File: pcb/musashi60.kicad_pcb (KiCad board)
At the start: 2 copper layers, 185 x 132 mm, 77 parts, among them J1 MJ-4PP-9, U1 ProMicro_r

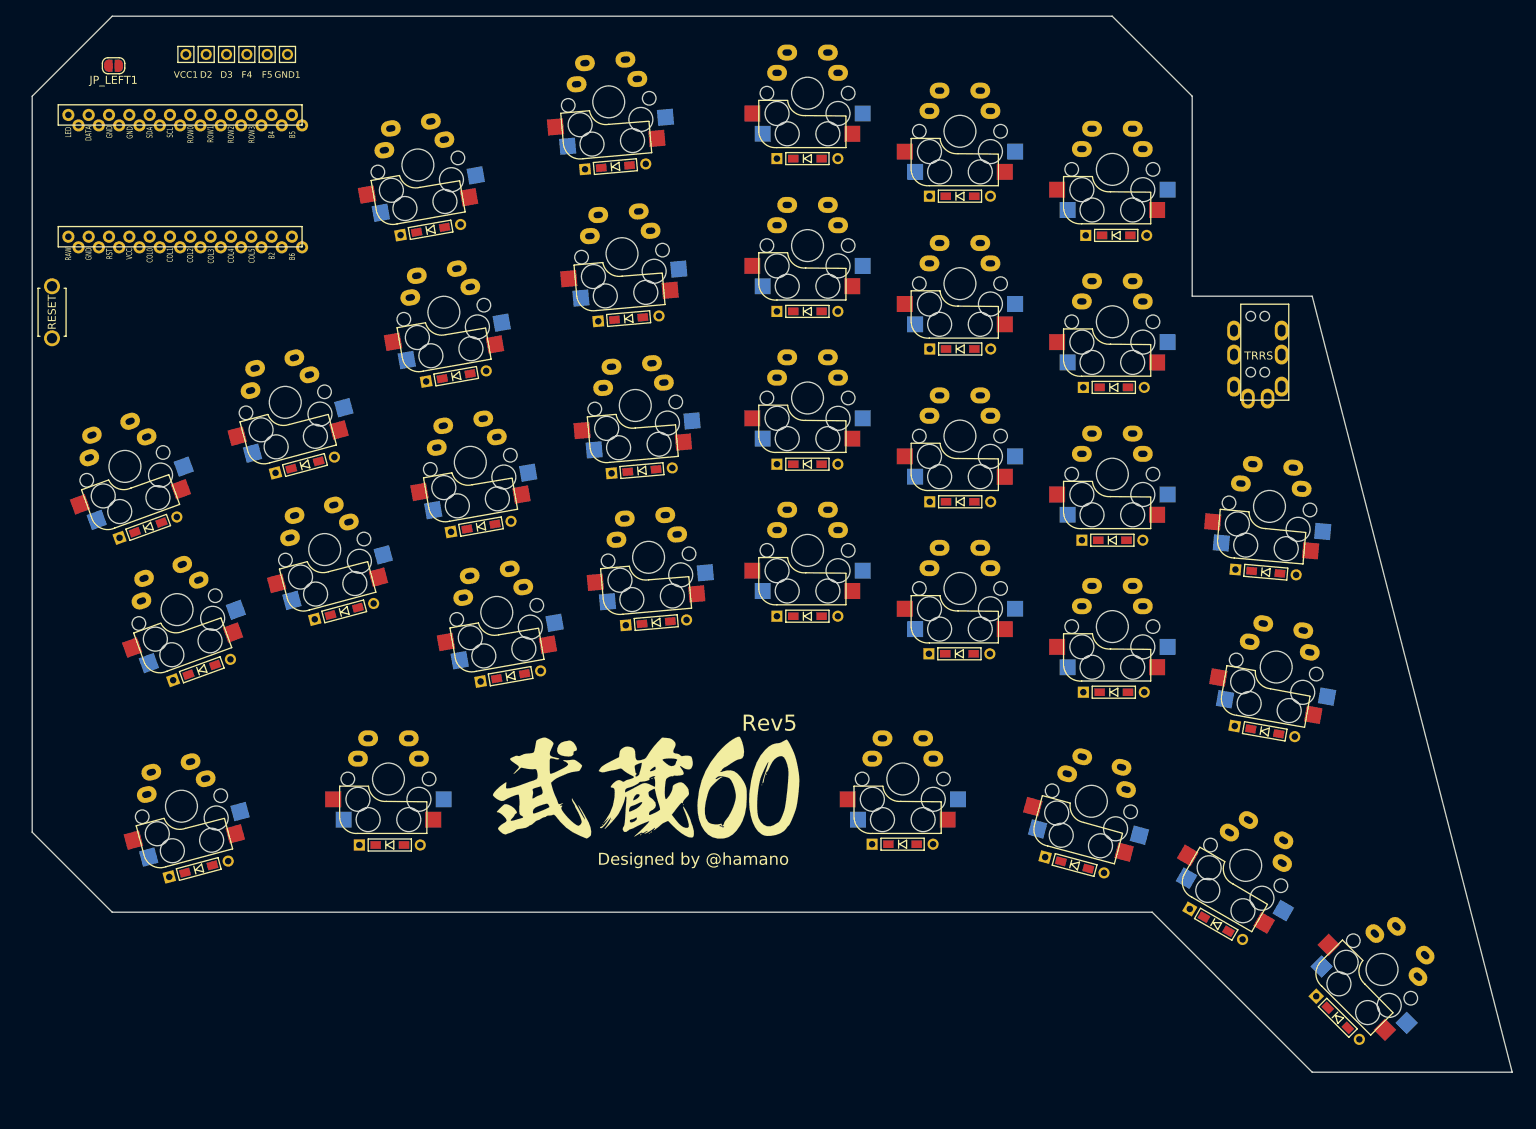
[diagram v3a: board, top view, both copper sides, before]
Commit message: update pcb
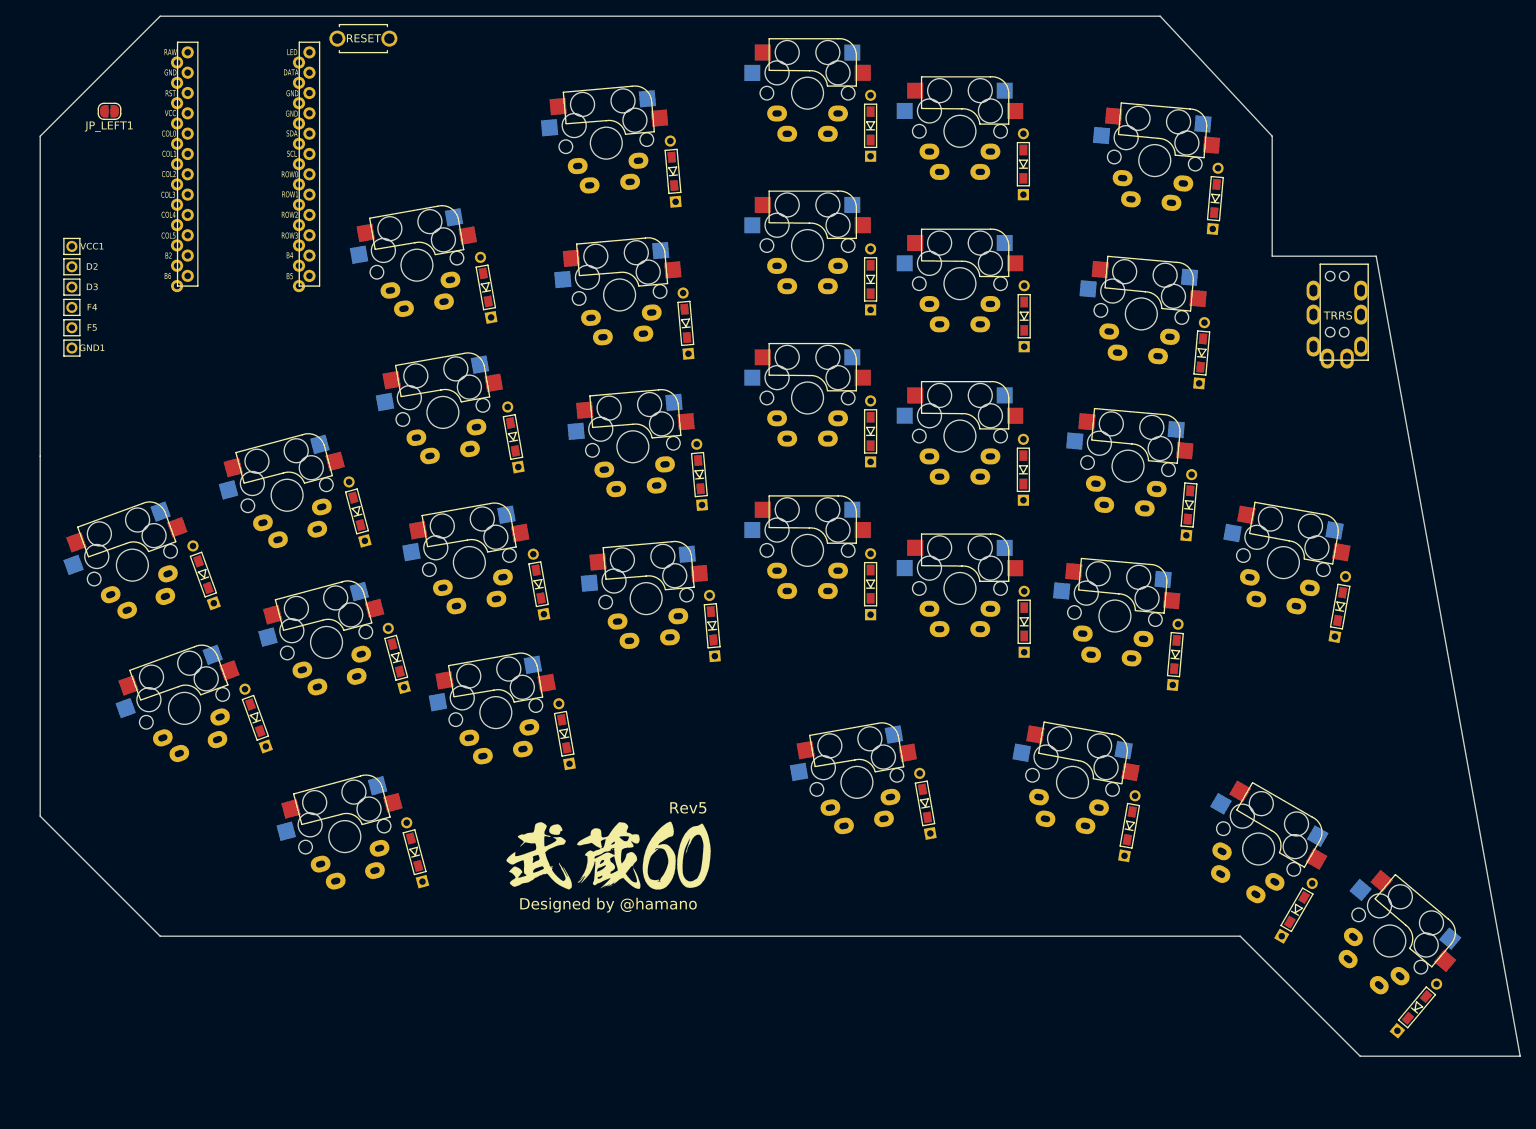
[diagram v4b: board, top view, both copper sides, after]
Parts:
- removed the D_A3 at (169.2, 82.5)
- removed D_H4: D, foostan:D3_TH_SMD
- removed the G_LOGO_B at (91.7, 109.4)
- removed the G_LOGO_F at (91.7, 109.5)
- removed the SW_A3 at (169.7, 74.3)
- removed SW_H4: SW_PUSH, local:CherryMX_Direct_Hotswap_Reversible
- added G_LOGO_B: LOGO, local:musashi60-silk-384, B.Cu at (87.0, 118.0)
- added G_LOGO_F: LOGO, local:musashi60-silk-384, F.Cu at (87.0, 118.0)
- moved SW_RST1 51.8 mm to (56.4, 15.8), turned to 0 degrees
- moved GND1 45.5 mm to (20.0, 54.5)
- moved F5 42.0 mm to (20.0, 51.9)
- moved F4 38.4 mm to (20.0, 49.4)
- moved D3 34.9 mm to (20.0, 46.9)
- moved D2 31.4 mm to (20.0, 44.3)
- moved VCC1 27.9 mm to (20.0, 41.8)
- moved D_A5 18.2 mm to (178.5, 86.8), turned to 80 degrees
- moved D_A1 13.2 mm to (162.9, 35.8), turned to 85 degrees
- moved SW_A5 13.1 mm to (171.4, 81.3)
- moved SW_E4 12.5 mm to (73.0, 100.0)
- moved SW_E1 12.5 mm to (63.1, 44.1)
- moved SW_E2 12.5 mm to (66.3, 62.5)
- moved SW_E3 12.5 mm to (69.6, 81.3)
- moved SW_G2 12.4 mm to (27.5, 81.6)
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- renumbered D_B1 to D_A1, D_B2 to D_A2, D_B3 to D_A3, D_B4 to D_A4, D_A4 to D_A5, D_C1 to D_B1, D_C2 to D_B2, D_C3 to D_B3, D_C4 to D_B4, D_A5 to D_B5, D_D1 to D_C1, D_D2 to D_C2, D_D3 to D_C3, D_D4 to D_C4, D_B5 to D_C5, D_E1 to D_D1, D_E2 to D_D2, D_E3 to D_D3, D_E4 to D_D4, D_C5 to D_D5, D_F1 to D_E1, D_F2 to D_E2, D_F3 to D_E3, D_F4 to D_E4, D_D5 to D_E5, D_G2 to D_F2, D_G3 to D_F3, D_G4 to D_F5, D_H2 to D_G2, D_H3 to D_G3, SW_B1 to SW_A1, SW_B2 to SW_A2, SW_B3 to SW_A3, SW_B4 to SW_A4, SW_A4 to SW_A5, SW_C1 to SW_B1, SW_C2 to SW_B2, SW_C3 to SW_B3, SW_C4 to SW_B4, SW_A5 to SW_B5, SW_D1 to SW_C1, SW_D2 to SW_C2, SW_D3 to SW_C3, SW_D4 to SW_C4, SW_B5 to SW_C5, SW_E1 to SW_D1, SW_E2 to SW_D2, SW_E3 to SW_D3, SW_E4 to SW_D4, SW_C5 to SW_D5, SW_F1 to SW_E1, SW_F2 to SW_E2, SW_F3 to SW_E3, SW_F4 to SW_E4, SW_D5 to SW_E5, SW_G2 to SW_F2, SW_G3 to SW_F3, SW_G4 to SW_F5, SW_H2 to SW_G2, SW_H3 to SW_G3
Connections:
- D_A5 pad 1: B3 -> B2
- D_C3 pad 2: Net-(D_D3-Pad2) (its old number) -> F7
- D_D2 pad 1: F7 -> Net-(D_D2-Pad1)
- D_E2 pad 1: F7 -> Net-(D_D2-Pad1)
- D_F2 pad 1: F7 -> Net-(D_D2-Pad1)
- D_F5 pad 1: B3 -> B2
- D_G2 pad 1: F7 -> Net-(D_D2-Pad1)
- SW_A1 pad 1: D0 -> D1
- SW_A2 pad 1: D0 -> D1
- SW_A3 pad 1: D0 -> D1
- SW_A4 pad 1: D0 -> D1
- SW_B1 pad 1: D4 -> D0
- SW_B2 pad 1: D4 -> D0
- SW_B3 pad 1: D4 -> D0
- SW_B4 pad 1: D4 -> D0
- SW_B5 pad 1: D1 -> D0
- SW_C1 pad 1: C6 -> D4
- SW_C2 pad 1: C6 -> D4
- SW_C3 pad 1: C6 -> D4
- SW_C3 pad 2: Net-(D_D3-Pad2) (its old number) -> F7
- SW_C4 pad 1: C6 -> D4
- SW_C5 pad 1: D0 -> D4
- SW_D1 pad 1: D7 -> C6
- SW_D2 pad 1: D7 -> C6
- SW_D3 pad 1: D7 -> C6
- SW_D4 pad 1: D7 -> C6
- SW_D5 pad 1: D4 -> C6
- SW_E1 pad 1: E6 -> D7
- SW_E2 pad 1: E6 -> D7
- SW_E3 pad 1: E6 -> D7
- SW_E4 pad 1: E6 -> D7
- SW_E5 pad 1: C6 -> D7
- SW_F2 pad 1: B4 -> E6
- SW_F3 pad 1: B4 -> E6
- SW_F5 pad 1: B4 -> E6
- SW_G2 pad 1: B5 -> B4
- SW_G3 pad 1: B5 -> B4
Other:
- board size 185 x 132 mm -> 185 x 130 mm
